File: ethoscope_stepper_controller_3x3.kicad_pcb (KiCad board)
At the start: 2 copper layers, 74.9 x 74.9 mm, 69 parts, among them P1 PWR_JACK_2.1x5.5_SMD_VERT, T1 TERM_BLK_HDR_4POS_VERT_0.138IN, T2 TERM_BLK_HDR_4POS_VERT_0.138IN, T3 TERM_BLK_HDR_4POS_VERT_0.138IN, T4 TERM_BLK_HDR_4POS_VERT_0.138IN, T5 TERM_BLK_HDR_4POS_VERT_0.138IN, T6 TERM_BLK_HDR_4POS_VERT_0.138IN, T7 TERM_BLK_HDR_4POS_VERT_0.138IN, U1 TMC429, U10 DRV8846, U11 TMC429, U12 BUFFER_TRI_STATE, U13 DRV8846, U2 BUFFER_TRI_STATE, U3 DRV8846, U4 DRV8846, U5 DRV8846, U6 TMC429, U7 BUFFER_TRI_STATE, U8 DRV8846, U9 DRV8846

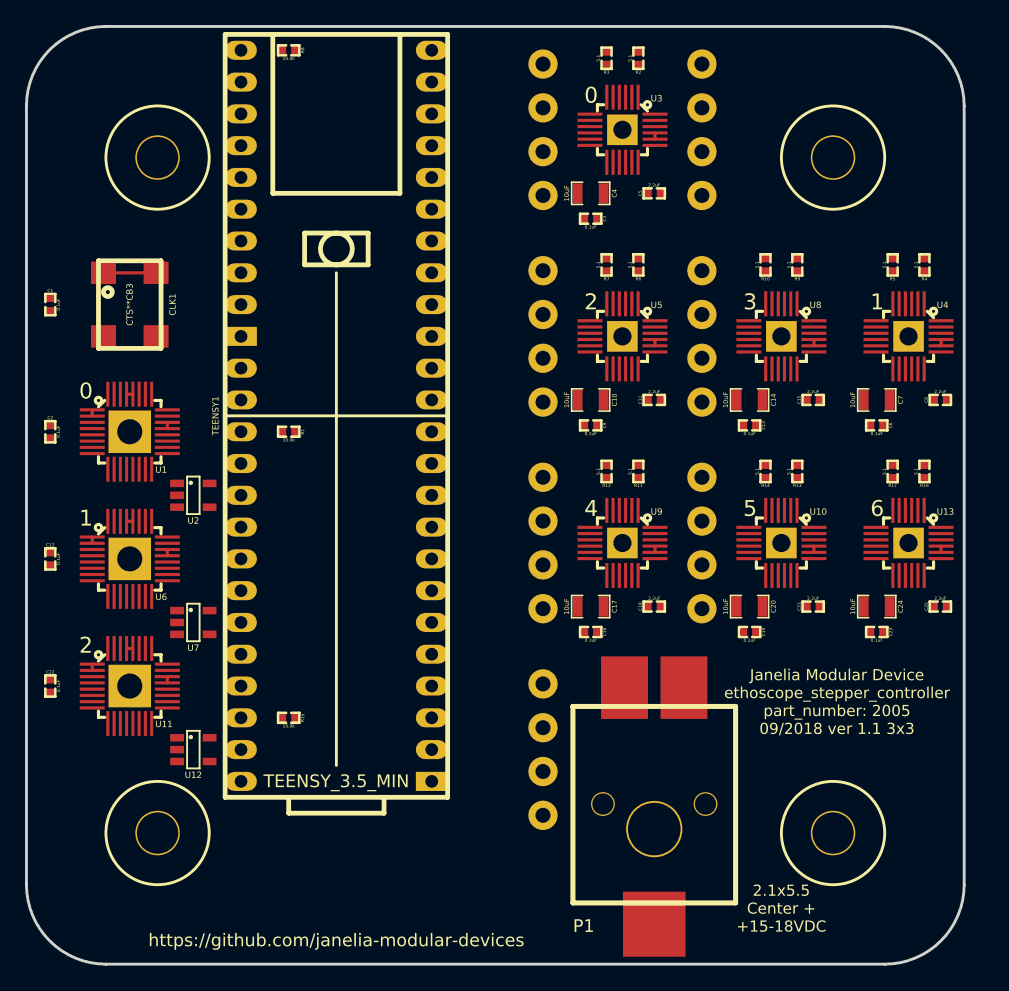
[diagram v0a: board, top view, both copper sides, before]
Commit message: Finished autorouting.
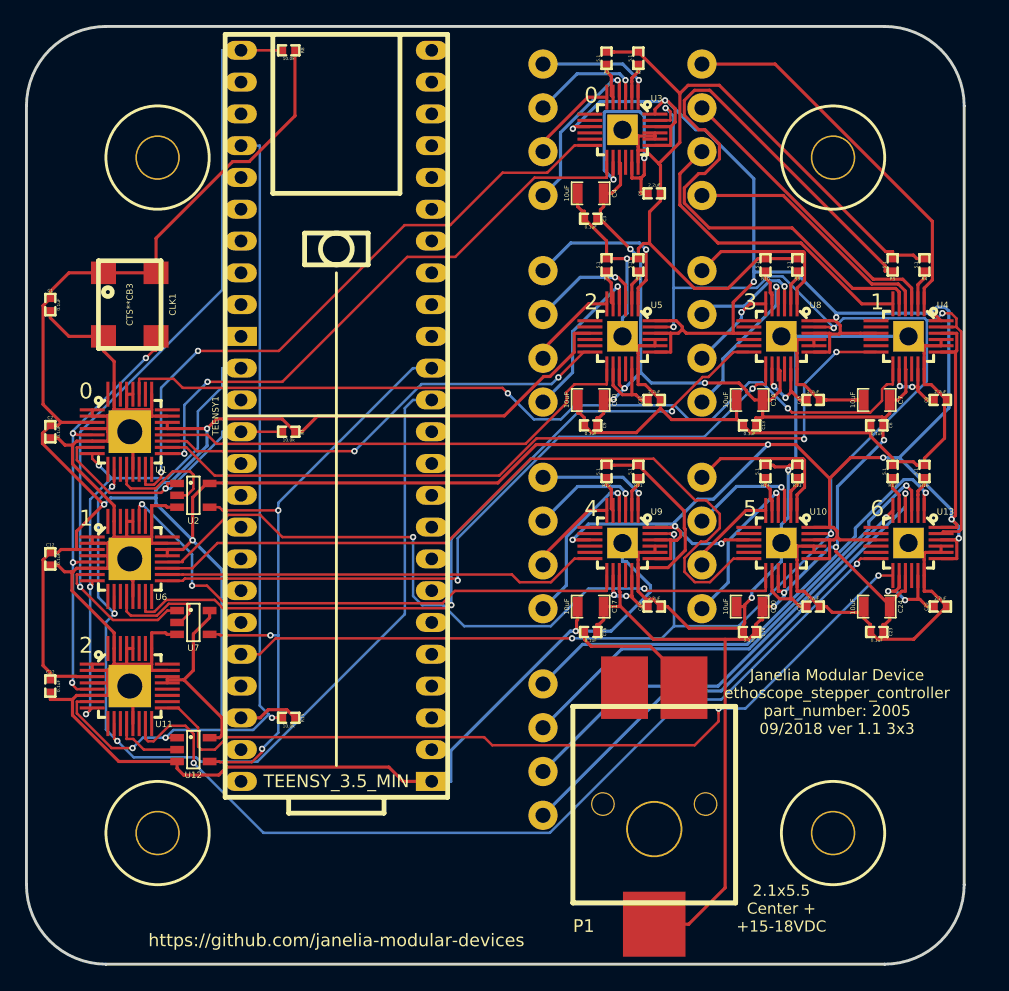
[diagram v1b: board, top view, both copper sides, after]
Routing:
- net GND: track 6.50 -> 441.3 mm, vias 0 -> 4
- net +3V3: track 5.70 -> 415.5 mm, vias 0 -> 15
- net /~SLEEP: track 0.00 -> 150.4 mm, vias 0 -> 7
- net VAA: track 0.00 -> 140.2 mm, vias 0 -> 8
- net /ethoscope_3x3/tmc_429_2/STEP_0: track 0.00 -> 74.3 mm, vias 0 -> 2
- net /MOSI: track 0.00 -> 73.8 mm, vias 0 -> 3
- net /~CS_429_2: track 0.00 -> 69.1 mm, vias 0 -> 3
- net /ethoscope_3x3/tmc429_0/DIR_1: track 0.00 -> 68.7 mm, vias 0 -> 2
- net /ethoscope_3x3/tmc_429_2/DIR_0: track 0.00 -> 67.1 mm, vias 0 -> 2
- net /ethoscope_3x3/tmc429_0/STEP_1: track 0.00 -> 64.3 mm, vias 0 -> 2
- net /~CS_429_1: track 0.00 -> 63.9 mm, vias 0 -> 1
- net /ethoscope_3x3/tmc429_1/STEP_2: track 0.00 -> 61.9 mm
- net /ethoscope_3x3/tmc429_1/STEP_0: track 0.00 -> 61.9 mm, vias 0 -> 2
- net /ethoscope_3x3/tmc429_1/DIR_2: track 0.00 -> 58.5 mm, vias 0 -> 2
- net /ethoscope_3x3/tmc429_1/DIR_0: track 0.00 -> 57.7 mm, vias 0 -> 2
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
